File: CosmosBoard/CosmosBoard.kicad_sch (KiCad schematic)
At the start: 36 parts, among them J1 VIN, J12 Conn_01x25, J2 USB_B_Micro, J3 power_jumper, J4 Conn_01x25, P1 SWD, SW1 SW_SPDT, SW2 SW_Push, U1 STM32F405RGT6, U3 AMS1117-3.3, X1 8MHz 10ppm (X50328MSB2GI), Y1 32.768

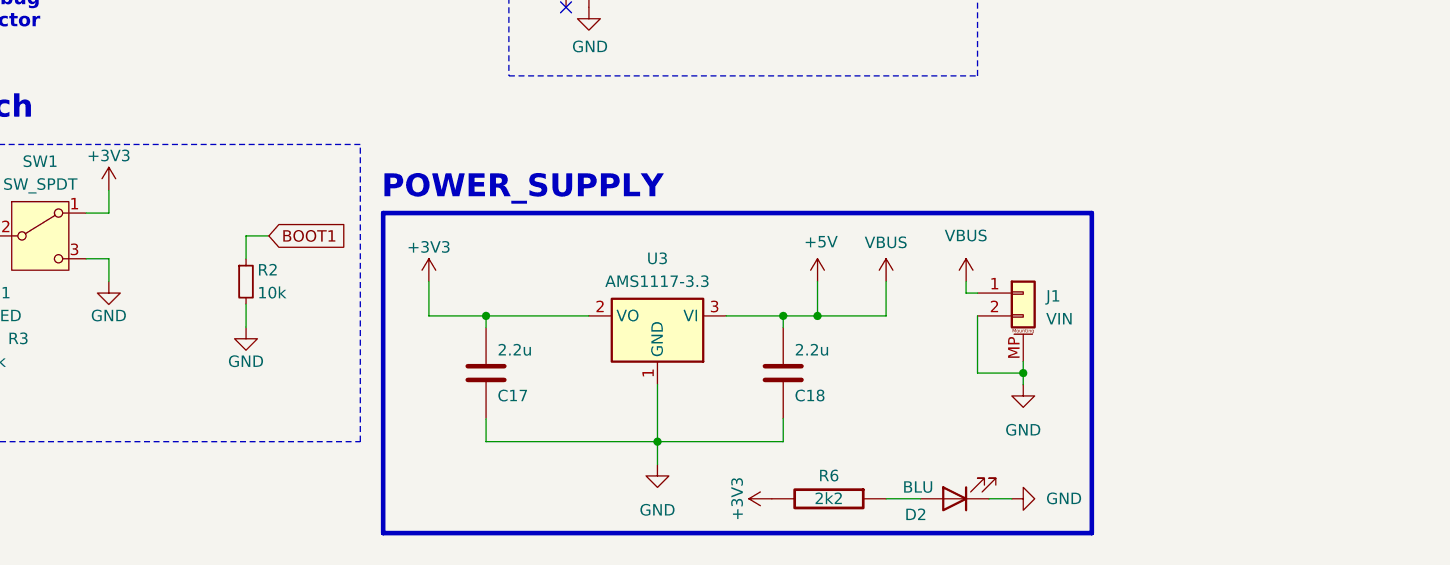
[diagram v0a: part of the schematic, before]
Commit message: traces
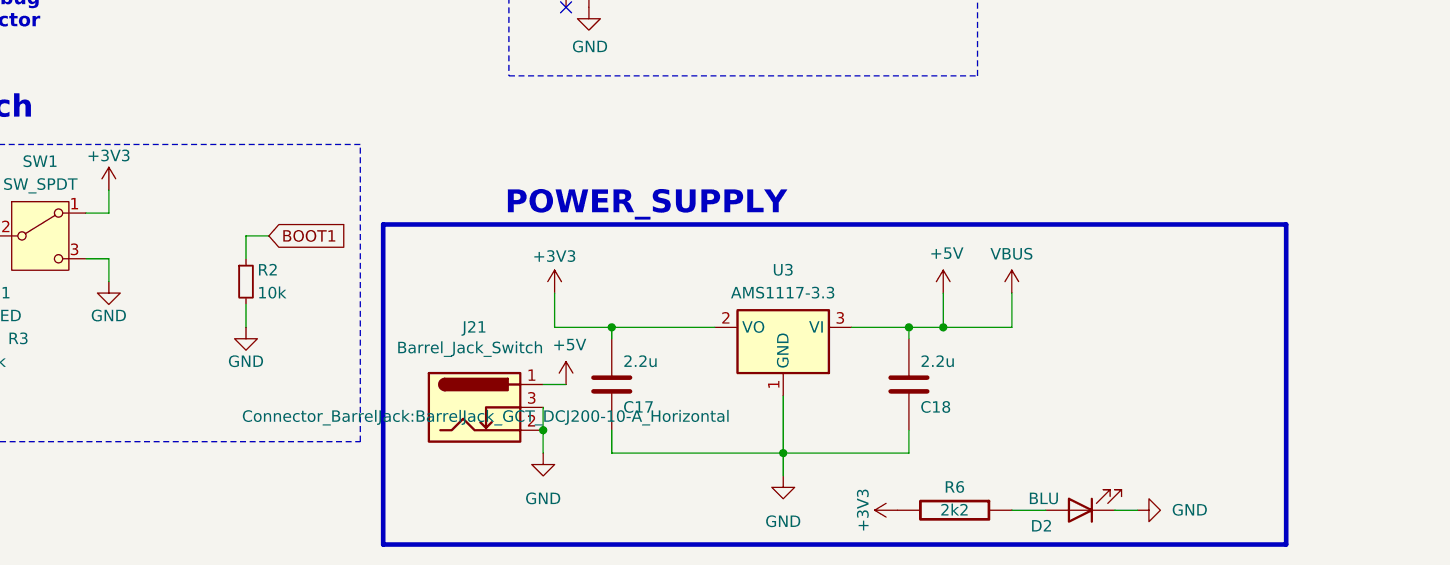
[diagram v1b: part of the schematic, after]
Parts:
- removed J1: VIN, Connector_JST:JST_GH_SM02B-GHS-TB_1x02-1MP_P1.25mm_Horizontal, symbol Connector_Generic_MountingPin:Conn_01x02_MountingPin
- added J21: Barrel_Jack_Switch, Connector_BarrelJack:BarrelJack_GCT_DCJ200-10-A_Horizontal, symbol Connector:Barrel_Jack_Switch
- SW2: footprint Button_Switch_THT:SW_PUSH-12mm -> Button_Switch_SMD:SW_Push_SPST_NO_Alps_SKRK
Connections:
- net +5V: now also J21.1
- net GND: now also J21.2, J21.3
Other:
- moved on the sheet: C17, C18, D2, R6, U3
